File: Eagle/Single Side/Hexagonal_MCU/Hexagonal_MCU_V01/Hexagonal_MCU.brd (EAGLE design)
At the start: 49.7 x 44 mm, 35 parts, among them J3 USB-MINIB-5PIN, Y1 16MHz

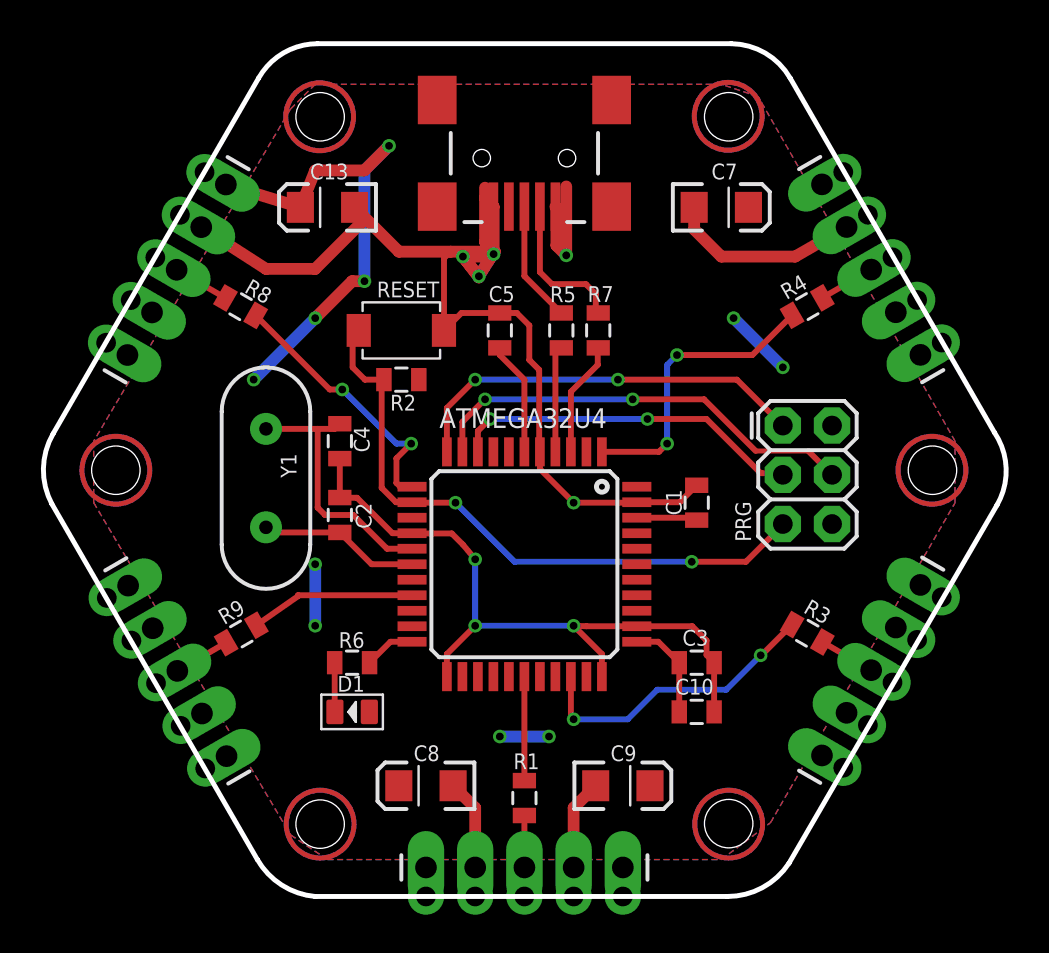
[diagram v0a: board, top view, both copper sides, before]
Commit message: Latest large panel designes
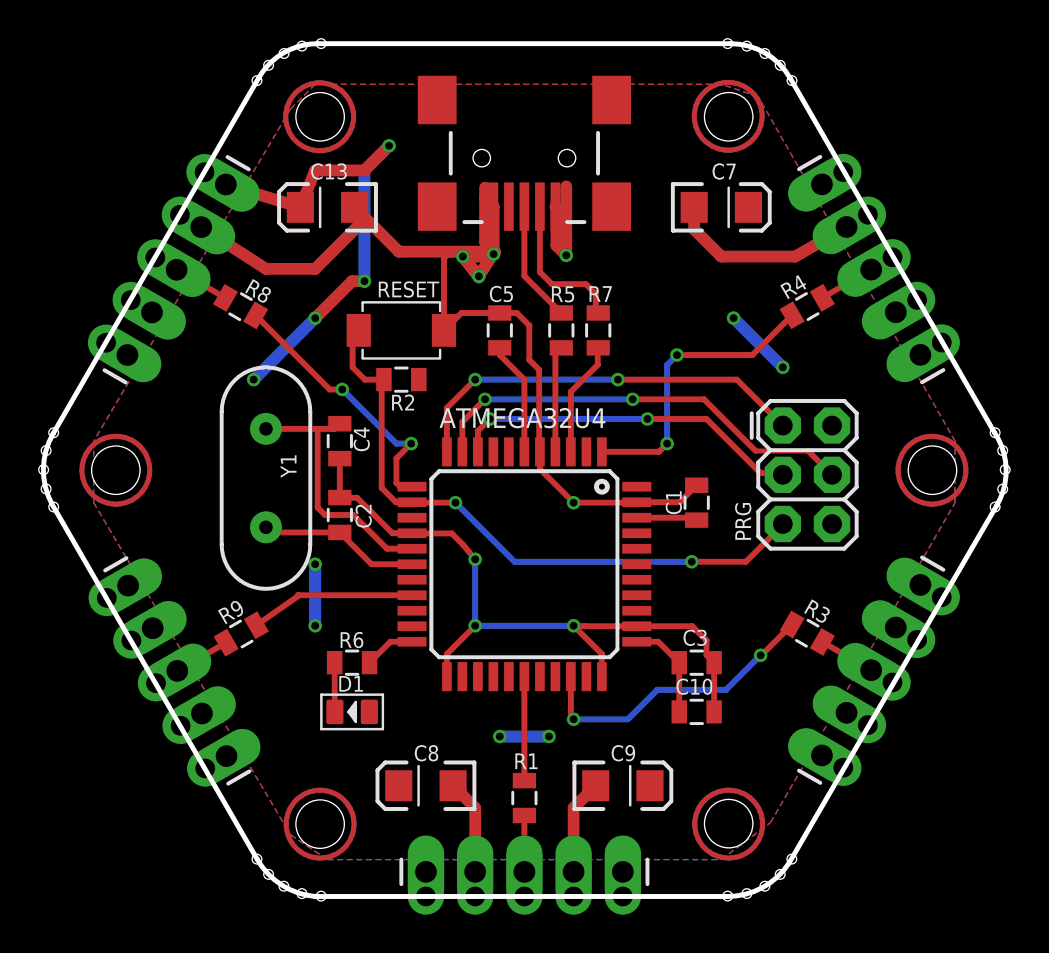
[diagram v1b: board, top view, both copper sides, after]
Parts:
- moved J4 0.23 mm to (30.5, 1.27)
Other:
- board text added: "ATMEGA32U4"
- board text added: "C1"
- board text added: "C10"
- board text added: "C13"
- board text added: "C2"
- board text added: "C3"
- board text added: "C4"
- board text added: "C5"
- board text added: "C7"
- board text added: "C8"
- board text added: "C9"
- board text added: "D1"
- board text added: "PRG"
- board text added: "R1"
- board text added: "R2"
- board text added: "R3"
- board text added: "R4"
- board text added: "R5"
- board text added: "R6"
- board text added: "R7"
- board text added: "R8"
- board text added: "R9"
- board text added: "RESET"
- board text added: "Y1"
